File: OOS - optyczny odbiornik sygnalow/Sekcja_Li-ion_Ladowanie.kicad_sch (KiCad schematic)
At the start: 18 parts, among them Q1 SI2301CDS-T1-GE3, Q2 AOSS32334C, Q3 AOSS32334C, U4 MCP73831-2-OT, U5 AP9101CAK6-ANTRG1, U6 AP2126K-ADJTRG1

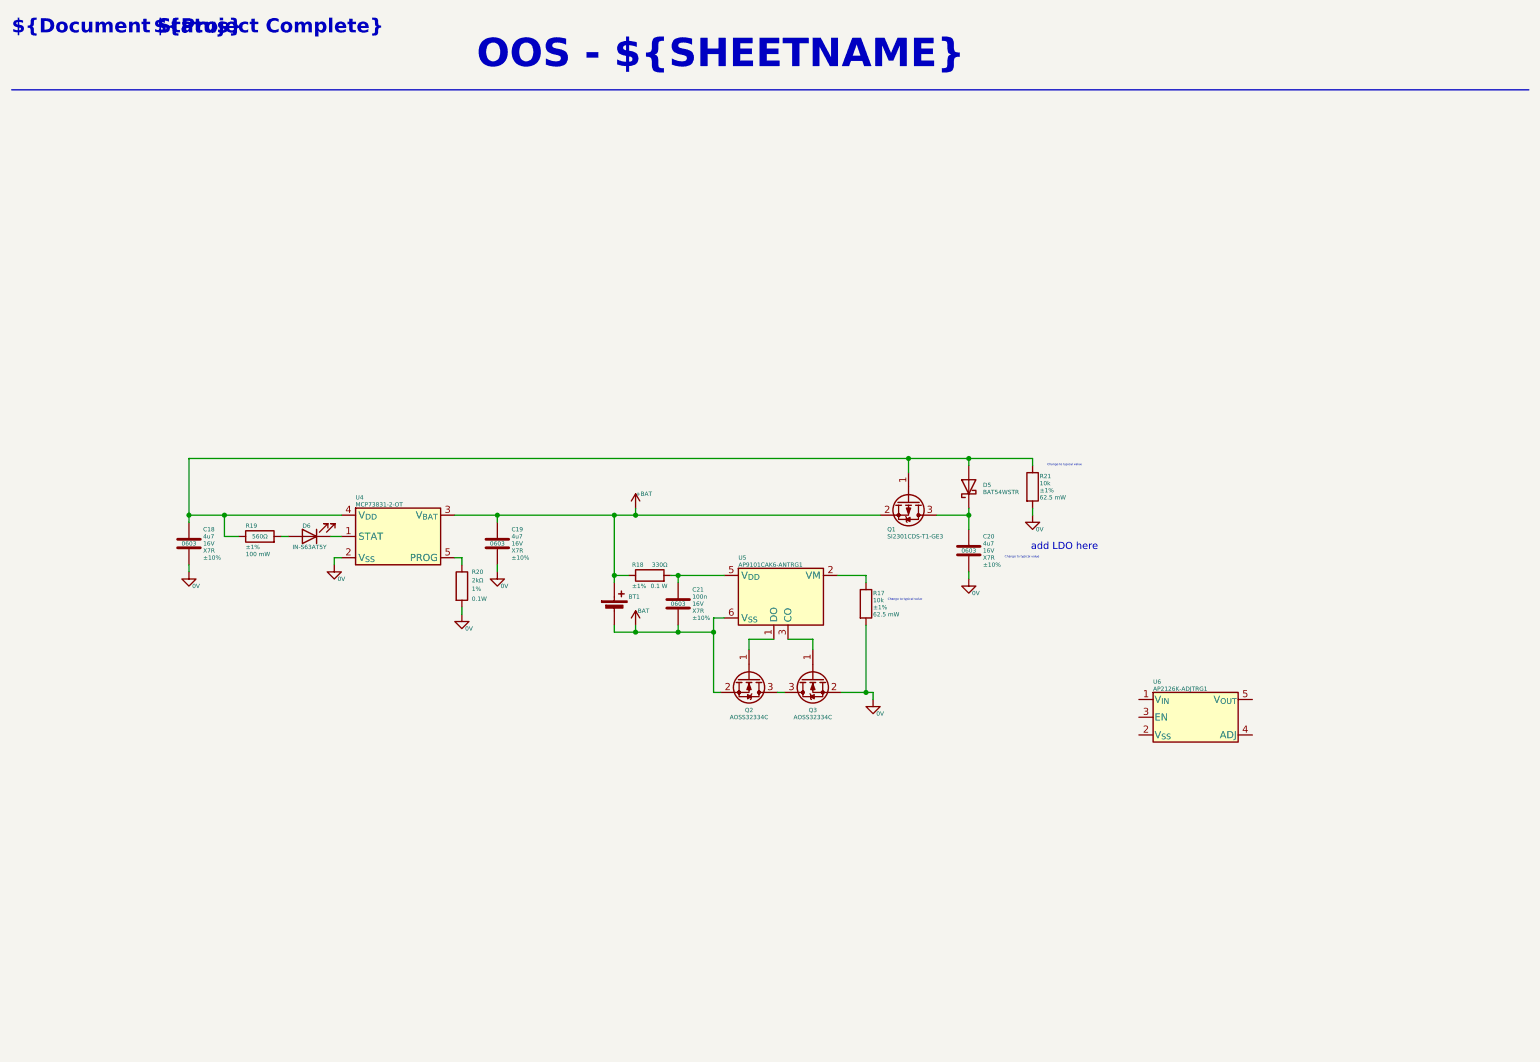
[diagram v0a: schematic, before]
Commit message: Finish Li-Lion section, add for review
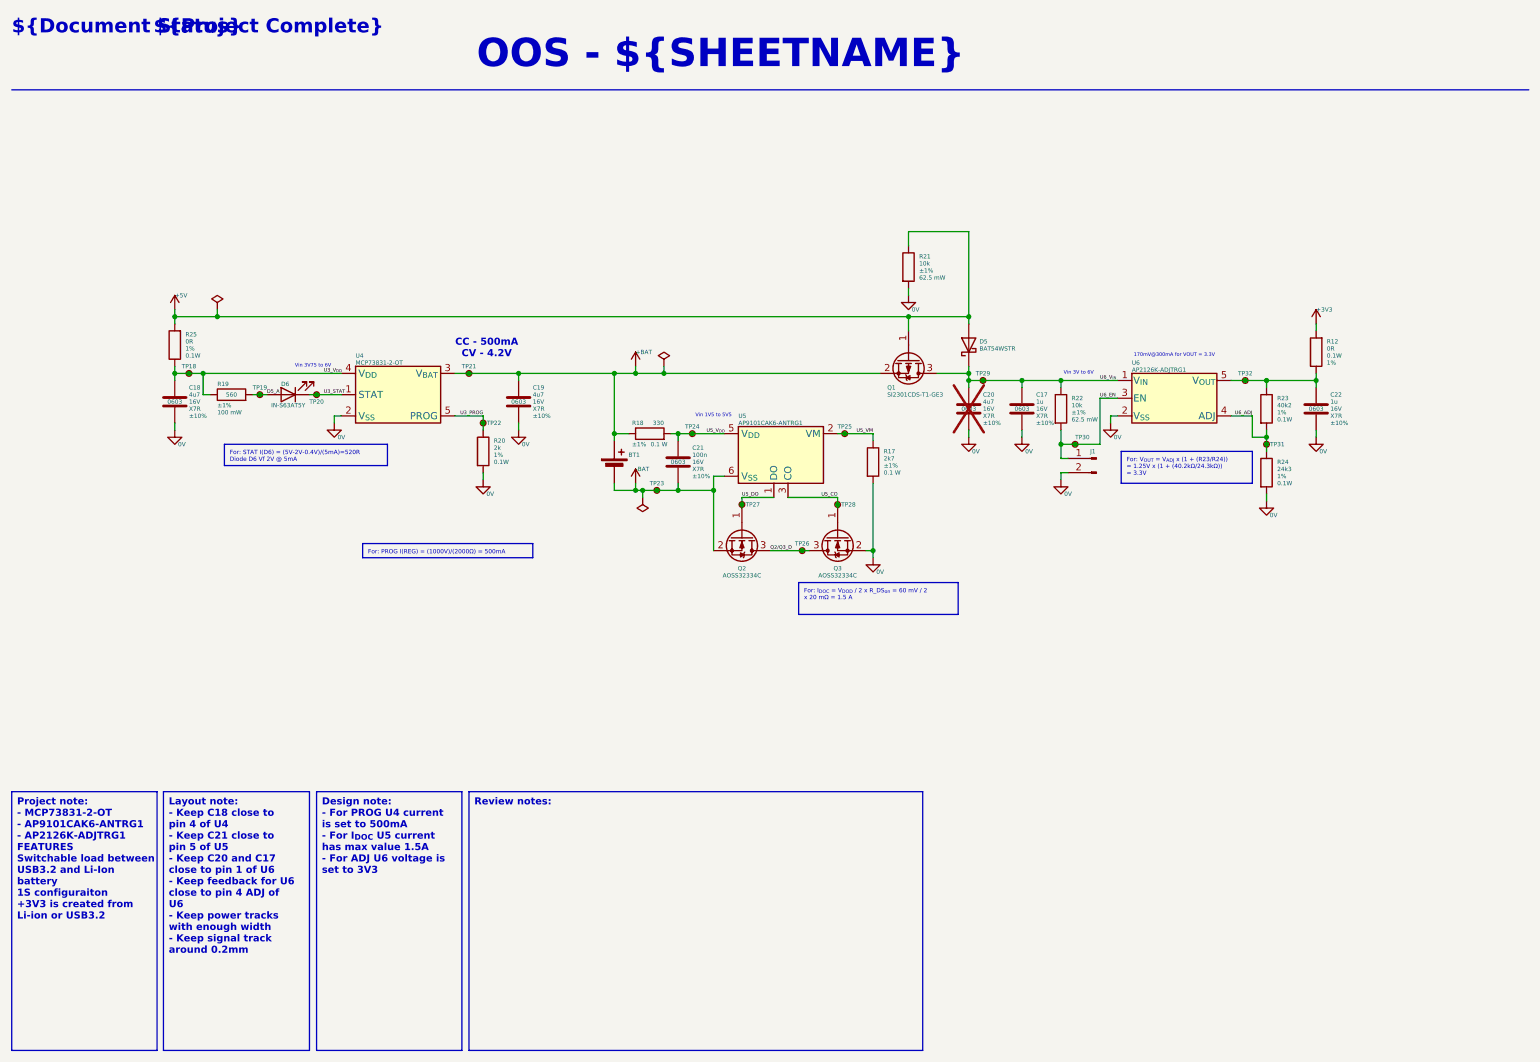
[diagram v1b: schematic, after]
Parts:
- added C17, C22: 1u, Capacitor_SMD:C_0603_1608Metric_Pad1.08x0.95mm_HandSolder, symbol Device:C
- added J1: Conn_01x02_Pin, Connector_PinHeader_2.54mm:PinHeader_1x02_P2.54mm_Vertical, symbol Connector:Conn_01x02_Pin
- added R12, R25: 0R, Resistor_SMD:R_0603_1608Metric, symbol Device:R
- added R22: 10k, Resistor_SMD:R_0402_1005Metric_Pad0.72x0.64mm_HandSolder, symbol Device:R
- added R23: 40k2, Resistor_SMD:R_0603_1608Metric, symbol Device:R
- added R24: 24k3, Resistor_SMD:R_0603_1608Metric, symbol Device:R
- added TP18, TP19, TP20, TP21, TP22, TP23, TP24, TP25, TP26, TP27, TP28, TP29, TP30, TP31, TP32: TestPoint_Small, TestPoint:TestPoint_Pad_D1.0mm, symbol Connector:TestPoint_Small
- C20: now not fitted
- Q2, Q3: Rds max (none) -> 26m; Rds typ (none) -> 20m
- R17: value 10k -> 2k7; footprint Resistor_SMD:R_0402_1005Metric_Pad0.72x0.64mm_HandSolder -> Resistor_SMD:R_0603_1608Metric_Pad0.98x0.95mm_HandSolder; MPN WR04X1002FTL -> ERJ3EKF2701V; Package 0402 -> 0603; Power Rating 62.5 mW -> 0.1 W; Supplier Link https://www.tme.eu/pl/details/wr04x1002ftl/rezystory-smd/wa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 -> https://www.tme.eu/pl/details/erj3ekf2701v/rezystory-smd/pa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
- R18: value 330Ω -> 330
- R19: value 560Ω -> 560
- R20: value 2kΩ -> 2k
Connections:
- net +BAT: now also TP21.1
- net -BAT: now also TP23.1
- net 0V: now also U6.2 (V_{SS}), C17.2, C22.2, J1.2 (Pin_2), R24.2
- net +5V: now reaches D5.2 (A), Q1.1 (G), R21.1
- net +5V: now also R25.2; no longer C18.1, R19.1, U4.4 (V_{DD})
- net D5_A: now reaches D6.2 (A), R19.2
- net D5_A: now also TP19.1
- net U6_V_{IN}: now reaches U6.1 (V_{IN})
- net U6_V_{IN}: now also C20.1, D5.1 (K), Q1.3 (D), C17.1, R22.1, TP29.1
- net U6_EN: now reaches U6.3 (EN)
- net U6_EN: now also J1.1 (Pin_1), R22.2, TP30.1
- net U6_ADJ: now reaches U6.4 (ADJ)
- net U6_ADJ: now also R23.2, R24.1, TP31.1
- net at U6.5 (V_{OUT}): now also C22.1, R12.1, R23.1, TP32.1
- net U5_VM: now reaches R17.1, U5.2 (VM)
- net U5_VM: now also TP25.1
- net U3_STAT: now reaches D6.1 (K), U4.1 (STAT)
- net U3_STAT: now also TP20.1
- net U3_PROG: now reaches R20.1, U4.5 (PROG)
- net U3_PROG: now also TP22.1
- net U5_DO: now reaches Q2.1 (G), U5.1 (DO)
- net U5_DO: now also TP27.1
- net U5_CO: now reaches Q3.1 (G), U5.3 (CO)
- net U5_CO: now also TP28.1
- net U5_V_{DD}: now reaches C21.1, R18.2, U5.5 (V_{DD})
- net U5_V_{DD}: now also TP24.1
- net Q2/Q3_D: now reaches Q2.3 (D), Q3.3 (D)
- net Q2/Q3_D: now also TP26.1
- new net +3V3: R12.2
- new net U3_V_{DD}: C18.1, R19.1, R25.1, TP18.1, U4.4 (V_{DD})
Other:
- note added: "170mV@300mA for VOUT = 3.3V"
- note added: "CC - 500mA CV - 4.2V"
- note added: "Vin 1V5 to 5V5"
- note added: "Vin 3V to 6V"
- note added: "Vin 3V75 to 6V"
- note removed: "Change to typical value"
- note removed: "add LDO here"
- moved on the sheet: BT1, C18, C19, C21, D5, D6, Q1, Q2, Q3, R17, R18, R19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

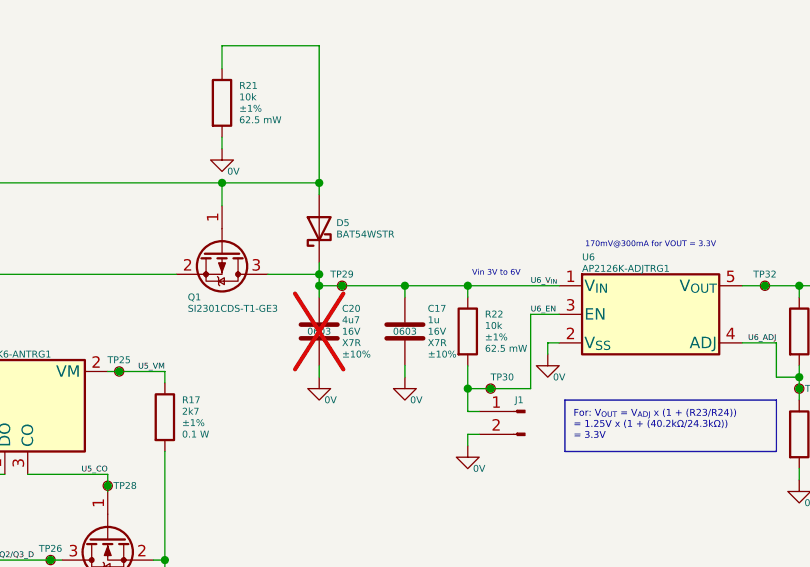
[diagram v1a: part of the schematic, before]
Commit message: Internal changes
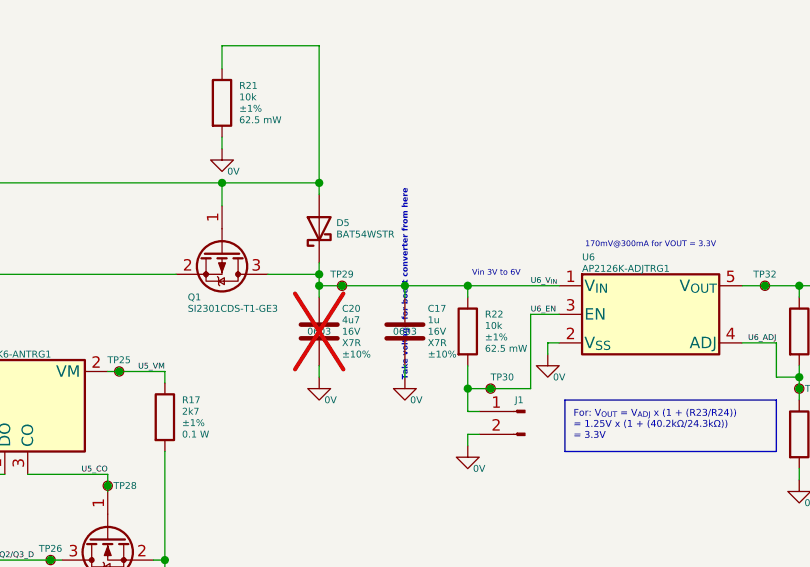
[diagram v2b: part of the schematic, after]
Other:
- note added: "Take voltage for boost converter from here"
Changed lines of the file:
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@@
+		)
+	)
+	(text "Take voltage for boost converter from here"
+		(exclude_from_sim no)
+		(at 193.675 77.47 90)
+		(effects
+			(font
+				(size 0.635 0.635)
+				(thickness 0.127)
+				(bold yes)
+				(color 255 0 0 1)
+			)
 		)
 	)
